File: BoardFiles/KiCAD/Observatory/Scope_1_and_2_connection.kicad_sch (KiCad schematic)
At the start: 0 parts

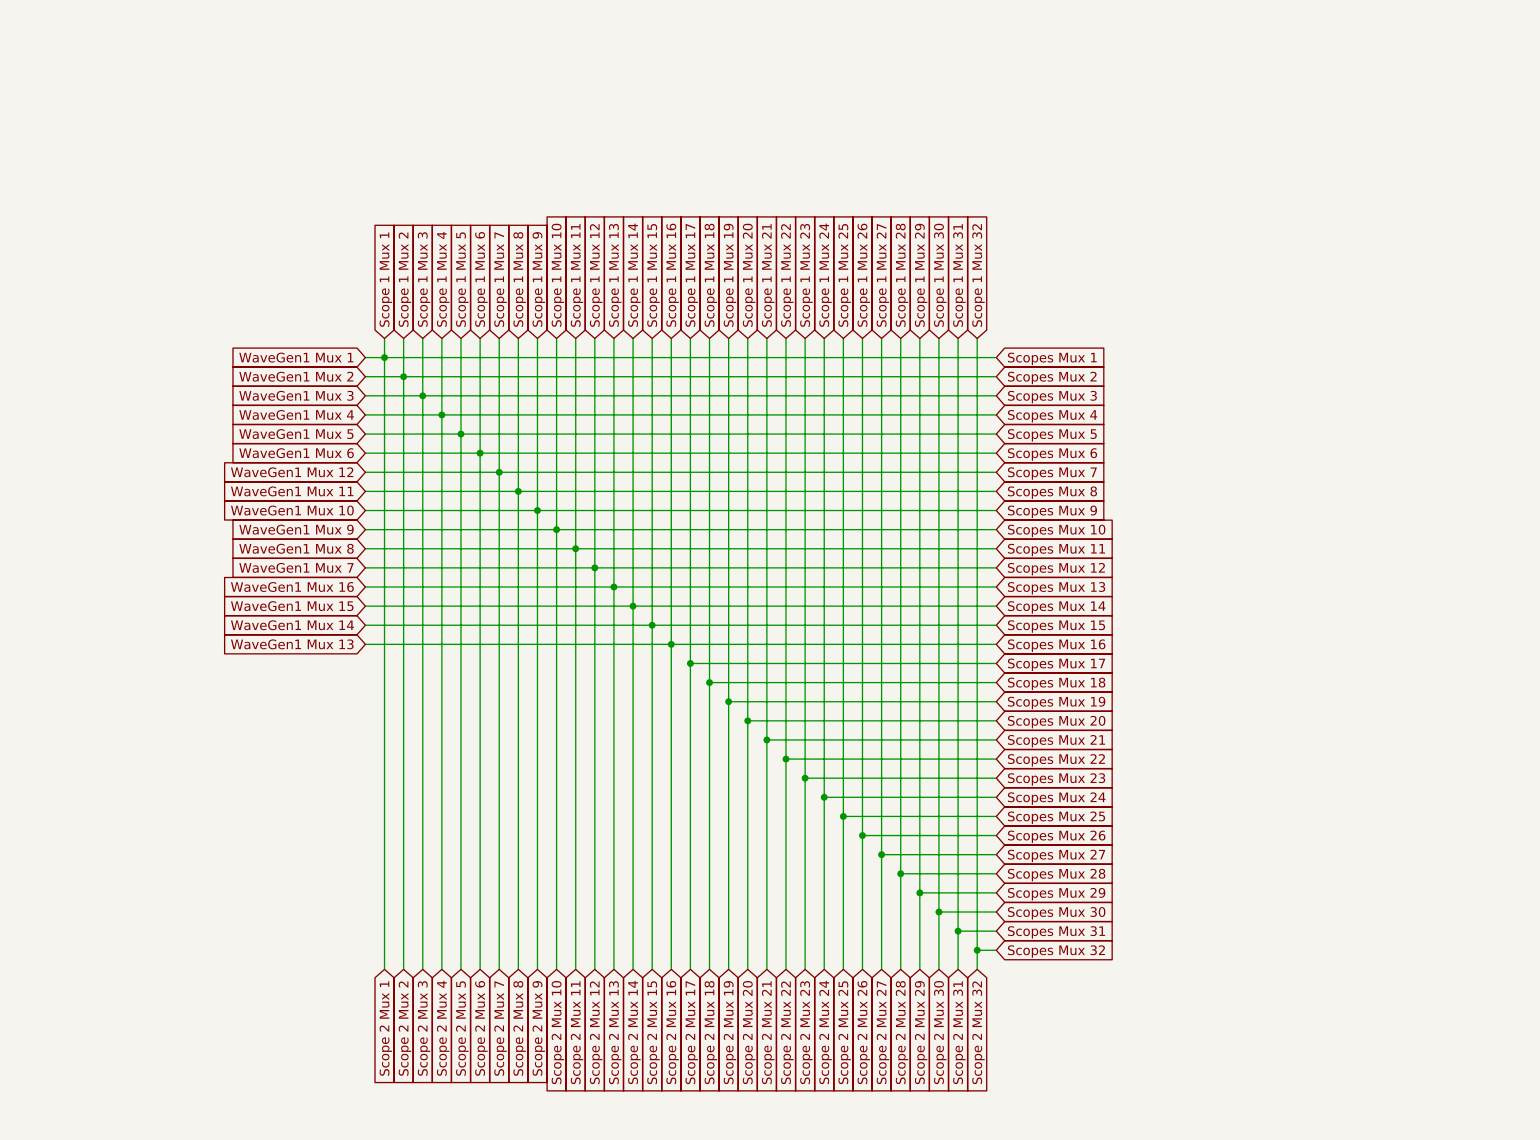
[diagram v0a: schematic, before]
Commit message: REV3 DRC pass
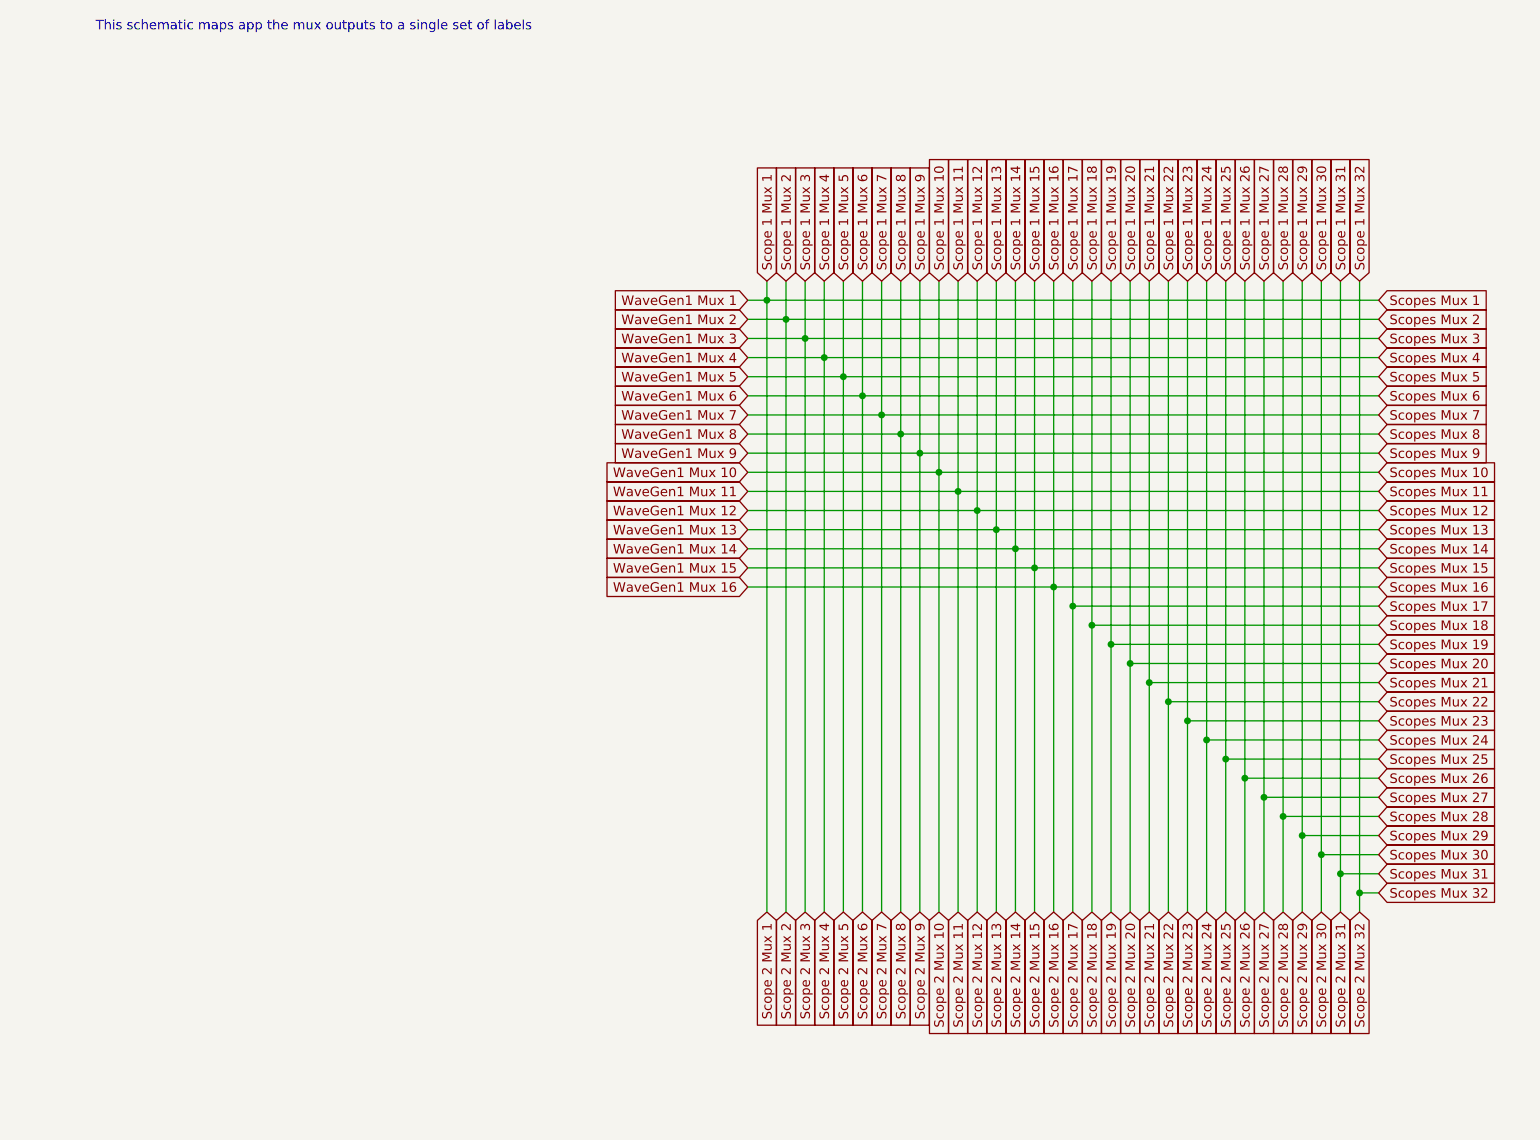
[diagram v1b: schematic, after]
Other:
- note added: "This schematic maps app the mux outputs to a single set of labels"
